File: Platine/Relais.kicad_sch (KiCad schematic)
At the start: 3 parts, among them K5 FINDER-40.41, Q5 BC547

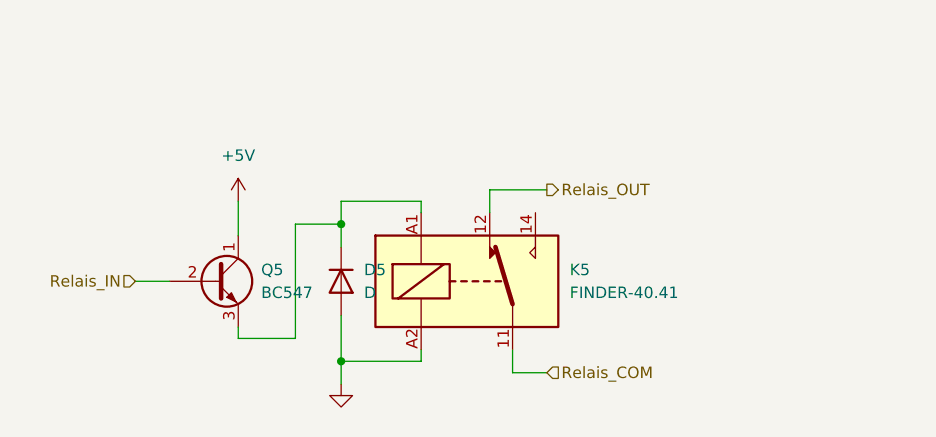
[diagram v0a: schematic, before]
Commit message: Platine fast fertig
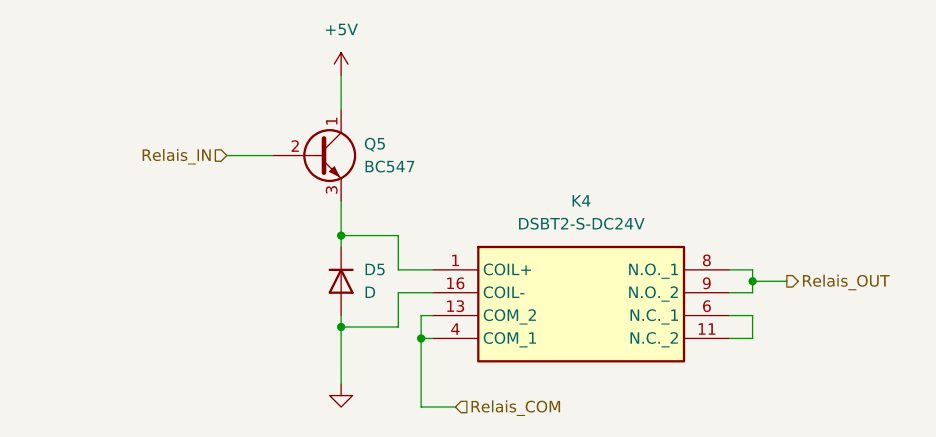
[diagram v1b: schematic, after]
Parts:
- removed K5: FINDER-40.41, Relay_THT:Relay_SPDT_Finder_40.41, symbol Relay:FINDER-40.41
- added K4: DSBT2-S-DC24V, DSBT2SDC24V, symbol BOH_KNX:DSBT2-S-DC24V
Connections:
- net GND: now also K4.16 (COIL-)
- net Relais_COM: now also K4.13 (COM_2), K4.4 (COM_1)
- net Relais_OUT: now also K4.8 (N.O._1), K4.9 (N.O._2)
- net at D5.1 (K), Q5.3 (E): now also K4.1 (COIL+)
- new net: K4.11 (N.C._2), K4.6 (N.C._1)
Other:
- moved on the sheet: Q5
